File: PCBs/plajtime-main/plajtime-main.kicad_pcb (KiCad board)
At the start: 6 copper layers, 15.2 x 34 mm, 82 parts, among them J1 RP SWD, J2 Internal connector, J3 Display connector, J4 Extention connector, J5 Conn_Coaxial, J6 Nordic SWD, J7 Conn_Coaxial, J8 Battery Connector, U1 W25Q64JWBYIM, U2 MP2664, U3 TPS628438YKA, U4 RP2350A, U5 BMA456, U6 MAX17055, U7 RV-3028-C7, U8 nRF52833_QDxx, U9 W25Q64JWU, Y1 13MHz, Y2 32MHz

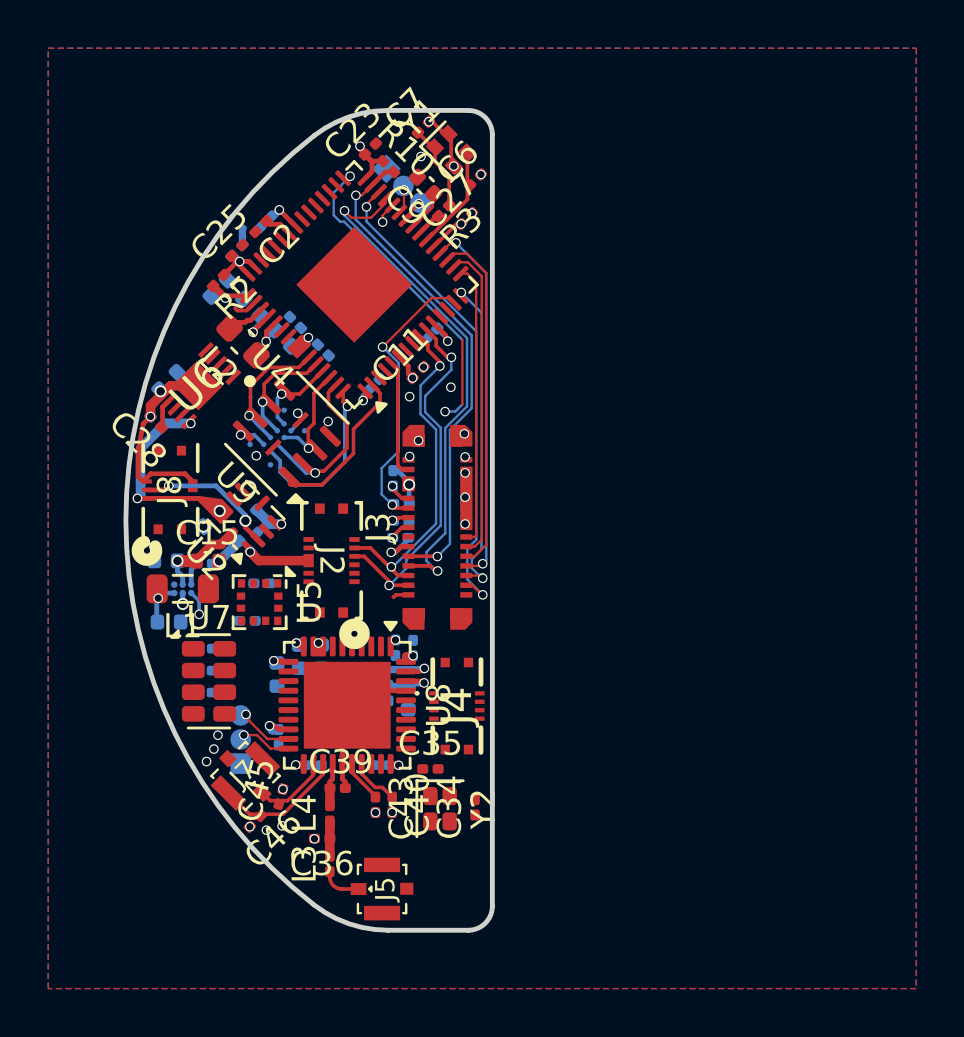
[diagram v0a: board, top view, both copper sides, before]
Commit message: Final?
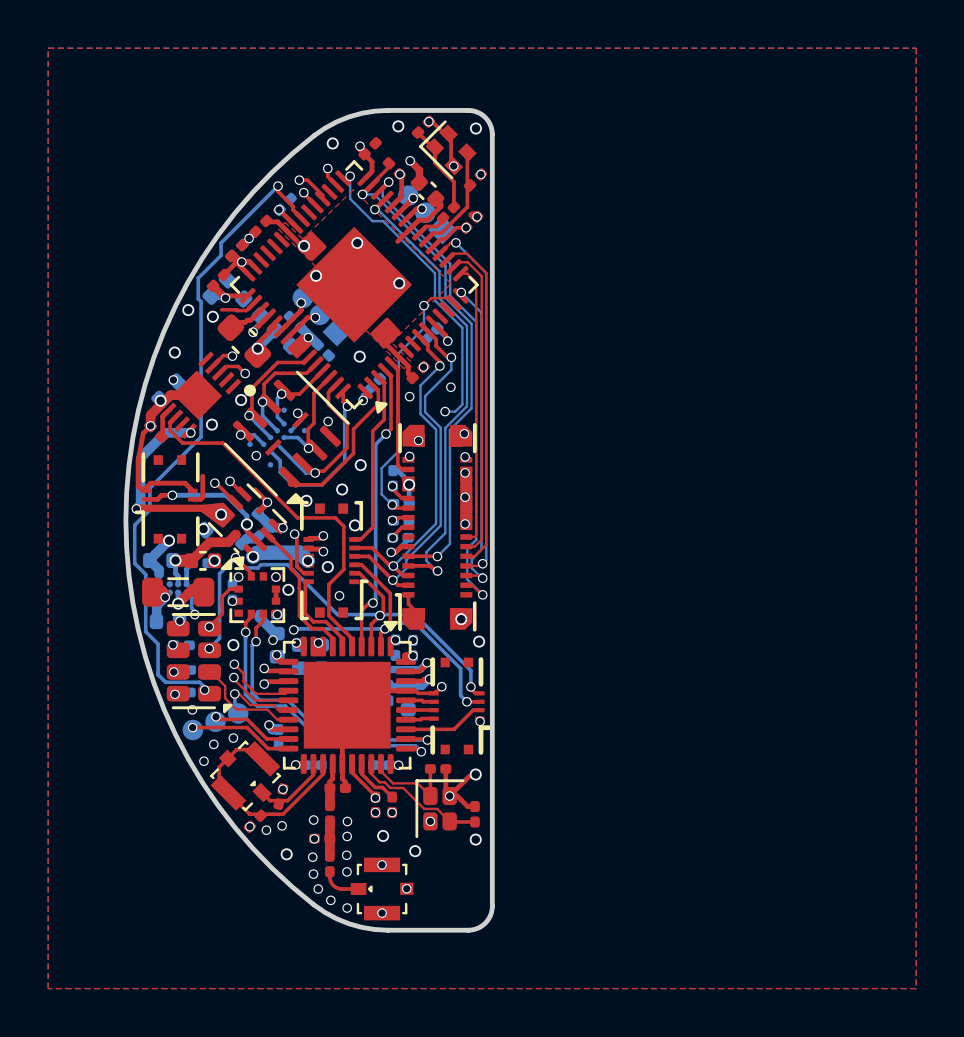
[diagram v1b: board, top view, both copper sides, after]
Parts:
- added J9: RP USB, Library:PinHeader_1x03_P1.00mm_Vertical, B.Cu at (44.0, 131.8)
- U3: footprint Package_BGA:Texas_DSBGA-6_0.757x1.01mm_Layout2x3_P0.35mm -> Library:Texas_DSBGA-6_0.757x1.01mm_Layout2x3_P0.35mm
- moved J1 3.44 mm to (48.4, 127.5), turned to 45 degrees
- moved R6 2.52 mm to (37.5, 144.8), turned to 0 degrees
- moved R5 2.40 mm to (37.6, 146.7), turned to 0 degrees
- moved J6 2.08 mm to (39.9, 147.6), turned to 110 degrees
- moved C30 1.54 mm to (37.6, 145.8)
- moved C29 1.27 mm to (39.6, 142.6), turned to 90 degrees
- moved C33 1.22 mm to (41.5, 144.8), turned to 90 degrees
- moved C22 1.09 mm to (41.8, 126.5), turned to 45 degrees
- moved U7 1.05 mm to (38.0, 145.4), turned to 180 degrees
- moved C24 0.93 mm to (41.1, 143.5), turned to 180 degrees
- moved J8 0.39 mm to (37.1, 138.7)
- moved C26 0.39 mm to (36.5, 135.9)
- moved C28 0.39 mm to (36.5, 135.9)
- moved R4 0.39 mm to (37.0, 134.2)
- moved U6 0.39 mm to (38.2, 134.4)
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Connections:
- C12 pad 1: +3.3V -> +3V
- C14 pad 1: +3.3V -> +3V
- C16 pad 1: +3.3V -> +3V
- C19 pad 1: +3.3V -> +3V
- C21 pad 1: +3.3V -> +3V
- C22 pad 1: +3.3V -> +3V
- C23 pad 1: +3.3V -> +3V
- C24 pad 1: +3.3V -> +3V
- C25 pad 1: +3.3V -> +3V
- C27 pad 1: +3.3V -> +3V
- C29 pad 1: +3.3V -> +3V
- C3 pad 1: +3.3V -> +3V
- C30 pad 2: +3.3V -> +3V
- C31 pad 1: +3.3V -> +3V
- C32 pad 1: +3.3V -> +3V
- C33 pad 1: +3.3V -> +3V
- C37 pad 1: +3.3V -> +3V
- C47 pad 1: +3.3V -> +3V
- J2 pad 2: SDA -> SCL
- J2 pad 3: SCL -> SDA
- J3 pad 11: +3.3V -> +3V
- J3 pad 23: +3.3V -> +3V
- J3 pad 25: +3.3V -> +3V
- J3 pad 29: +3.3V -> +3V
- J3 pad 30: +3.3V -> +3V
- J4 pad 1: +3.3V -> +3V
- J4 pad 2: SCL -> /EXT_INT
- J4 pad 3: /EXT_INT -> /EXT_GPIO_2
- J4 pad 4: SDA -> /EXT_RST
- J4 pad 5: /EXT_RST -> SDA
- J4 pad 6: unconnected-(J4-Pin_6-Pad6) -> /EXT_GPIO_1
- J4 pad 7: /EXT_GPIO -> SCL
- J6 pad 1: GND -> Net-(J6-Pin_1)
- R10 pad 1: +3.3V -> +3V
- R2 pad 1: +3.3V -> +3V
- R7 pad 1: +3.3V -> +3V
- R8 pad 1: +3.3V -> +3V
- R9 pad 1: +3.3V -> +3V
- U1 pad B2: +3.3V -> +3V
- U4 pad 1: +3.3V -> +3V
- U4 pad 11: +3.3V -> +3V
- U4 pad 20: +3.3V -> +3V
- U4 pad 24: Net-(J1-Pin_3) -> Net-(J1-Pin_2)
- U4 pad 25: Net-(J1-Pin_2) -> Net-(J1-Pin_3)
- U4 pad 26: +3.3V -> +3V
- U4 pad 3: unconnected-(U4-GPIO1-Pad3) -> /SLIDER_INT
- U4 pad 30: +3.3V -> +3V
- U4 pad 32: unconnected-(U4-GPIO20-Pad32) -> /VIC_INT
- U4 pad 36: /SLIDER_INT -> unconnected-(U4-GPIO24-Pad36)
- U4 pad 38: +3.3V -> +3V
- U4 pad 44: +3.3V -> +3V
- U4 pad 45: +3.3V -> +3V
- U4 pad 49: +3.3V -> +3V
- U4 pad 51: unconnected-(U4-USB_DM-Pad51) -> Net-(J9-Pin_3)
- U4 pad 52: unconnected-(U4-USB_DP-Pad52) -> Net-(J9-Pin_2)
- U4 pad 53: +3.3V -> +3V
- U4 pad 54: +3.3V -> +3V
- U5 pad 10: +3.3V -> +3V
- U5 pad 3: +3.3V -> +3V
- U5 pad 7: +3.3V -> +3V
- U6 pad 11: unconnected-(U6-CSP-Pad11) -> -BATT
- U7 pad 7: +3.3V -> +3V
- U8 pad 11: +3.3V -> +3V
- U8 pad 16: Net-(U8-P0.18/~{RESET}) -> Net-(J6-Pin_1)
- U8 pad 17: GPU_INT -> /RTC_INT
- U8 pad 18: +3.3V -> +3V
- U8 pad 19: Net-(J6-Pin_3) -> Net-(J6-Pin_2)
- U8 pad 20: Net-(J6-Pin_2) -> Net-(J6-Pin_3)
- U8 pad 30: +3.3V -> +3V
- U8 pad 31: /IMU_INT_2 -> /IMU_INT_1
- U8 pad 32: /IMU_INT_1 -> /IMU_INT_2
- U8 pad 33: /CHARGER_INT -> /EXT_GPIO_2
- U8 pad 36: /GAUGE_INT -> /EXT_GPIO_1
- U8 pad 4: unconnected-(U8-AIN2/P0.04-Pad4) -> GPU_INT
- U8 pad 40: +3.3V -> +3V
- U8 pad 5: unconnected-(U8-AIN3/P0.05-Pad5) -> /GAUGE_INT
- U8 pad 6: /RTC_INT -> /OXY_INT
- U8 pad 7: /OXY_INT -> /CHARGER_INT
- U8 pad 8: +3.3V -> +3V
- U8 pad 9: +3.3V -> +3V
- U9 pad 8: +3.3V -> +3V
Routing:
- net SDA: track 0.00 -> 35.4 mm, vias 0 -> 6
- net SCL: track 0.00 -> 32.3 mm, vias 0 -> 6
- net UART_TX: track 0.00 -> 30.4 mm, vias 0 -> 2
- net UART_RX: track 0.00 -> 28.9 mm, vias 0 -> 2
- net /CLK_OUT: track 0.00 -> 27.3 mm, vias 0 -> 2
- net +3V: track 1.80 -> 27.6 mm, vias 1 -> 25
- net +3.3V: track 23.2 -> 0.00 mm, vias 19 -> 0
- net /VIC_INT: track 0.00 -> 19.0 mm, vias 0 -> 2
- net /GAUGE_INT: track 0.00 -> 15.1 mm
- net /IMU_INT_2: track 0.00 -> 12.5 mm, vias 0 -> 2
- net /IMU_INT_1: track 0.00 -> 12.4 mm, vias 0 -> 2
- net USB_D-: track 0.00 -> 12.2 mm, vias 0 -> 2
- net GPU_INT: track 0.00 -> 12.1 mm, vias 0 -> 2
- net GND: track 11.6 -> 23.2 mm, vias 28 -> 80
- net USB_D+: track 0.00 -> 10.7 mm, vias 0 -> 2
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- added copper zone on F.Cu, net +1V1
- added copper zone on In2.Cu, net +3V
- removed copper zone on In2.Cu, net +3.3V
